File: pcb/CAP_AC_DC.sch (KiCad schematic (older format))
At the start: 6 parts

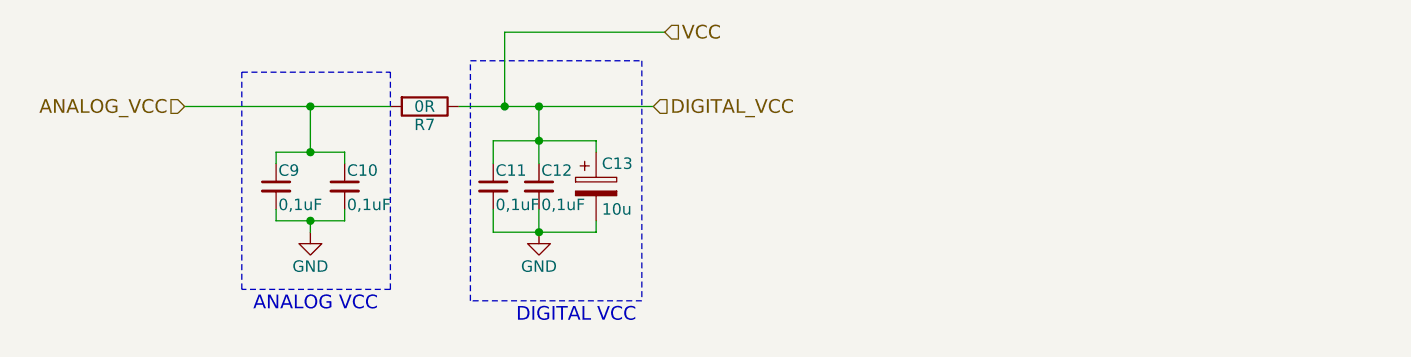
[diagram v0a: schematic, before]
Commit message: Clean up Kicad and TCC
Some changes in the
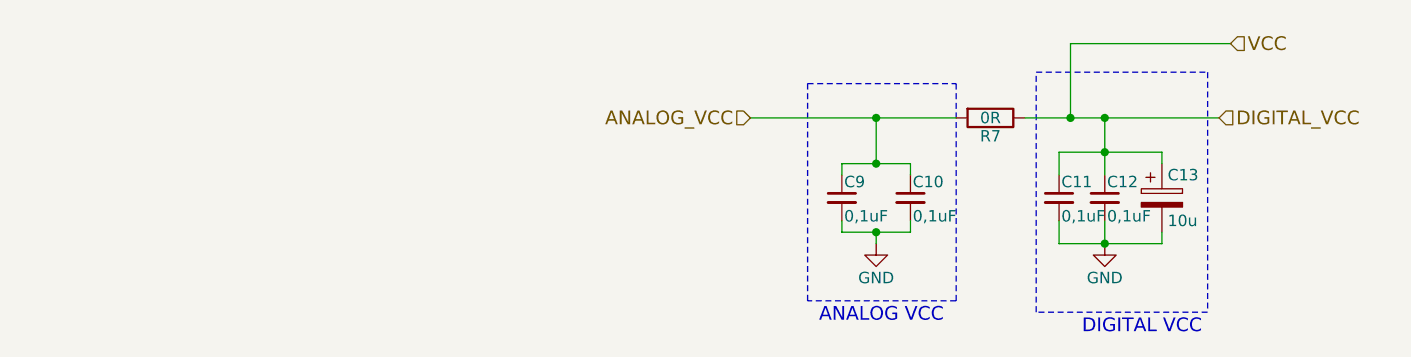
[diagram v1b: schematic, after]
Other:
- moved on the sheet: C10, C11, C12, C13, C9, R7
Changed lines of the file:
@@
 encoding utf-8
 Sheet 3 10
-Title ""
+Title "Capacitor Bank Schematic"
 Date ""
-Rev ""
-Comp ""
+Rev "1"
+Comp "Universidade de Brasília - Campus Gama"
 Comment1 ""
 Comment2 ""
@@
 L Device:C_Small C9
 U 1 1 5B1CC325
-P 3000 3650
-F 0 "C9" H 3010 3720 50  0000 L CNN
-F 1 "0,1uF" H 3010 3570 50  0000 L CNN
-F 2 "Capacitors_SMD:C_1206" H 3000 3650 50  0001 C CNN
-F 3 "https://www.digikey.com/product-detail/en/yageo/CC1206KRX7R9BB104/311-1179-1-ND/303089" H 3000 3650 50  0001 C CNN
-	1    3000 3650
+P 5475 3700
+F 0 "C9" H 5485 3770 50  0000 L CNN
+F 1 "0,1uF" H 5485 3620 50  0000 L CNN
+F 2 "Capacitors_SMD:C_1206" H 5475 3700 50  0001 C CNN
+F 3 "https://www.digikey.com/product-detail/en/yageo/CC1206KRX7R9BB104/311-1179-1-ND/303089" H 5475 3700 50  0001 C CNN
+	1    5475 3700
 	1    0    0    -1
 $EndComp
@@
 L Device:CP C13
 U 1 1 5B1CC377
-P 4400 3650
-F 0 "C13" H 4425 3750 50  0000 L CNN
-F 1 "10u" H 4425 3550 50  0000 L CNN
-F 2 "Capacitors_SMD:C_1206" H 4438 3500 50  0001 C CNN
-F 3 "https://www.digikey.com/product-detail/en/avx-corporation/TAJA106K006RNJ/478-1653-1-ND/564685" H 4400 3650 50  0001 C CNN
-	1    4400 3650
+P 6875 3700
+F 0 "C13" H 6900 3800 50  0000 L CNN
+F 1 "10u" H 6900 3600 50  0000 L CNN
+F 2 "Capacitors_SMD:C_1206" H 6913 3550 50  0001 C CNN
+F 3 "https://www.digikey.com/product-detail/en/avx-corporation/TAJA106K006RNJ/478-1653-1-ND/564685" H 6875 3700 50  0001 C CNN
+	1    6875 3700
 	1    0    0    -1
 $EndComp
@@
 L Device:C_Small C10
 U 1 1 5B1CC4B7
-P 3300 3650
-F 0 "C10" H 3310 3720 50  0000 L CNN
-F 1 "0,1uF" H 3310 3570 50  0000 L CNN
-F 2 "Capacitors_SMD:C_1206" H 3300 3650 50  0001 C CNN
-F 3 "https://www.digikey.com/product-detail/en/yageo/CC1206KRX7R9BB104/311-1179-1-ND/303089" H 3300 3650 50  0001 C CNN
-	1    3300 3650
+P 5775 3700
+F 0 "C10" H 5785 3770 50  0000 L CNN
+F 1 "0,1uF" H 5785 3620 50  0000 L CNN
+F 2 "Capacitors_SMD:C_1206" H 5775 3700 50  0001 C CNN
+F 3 "https://www.digikey.com/product-detail/en/yageo/CC1206KRX7R9BB104/311-1179-1-ND/303089" H 5775 3700 50  0001 C CNN
+	1    5775 3700
 	1    0    0    -1
 $EndComp
 Wire Wire Line
-	3000 3550 3000 3500
+	5475 3600 5475 3550
 Wire Wire Line
-	3000 3500 3150 3500
+	5475 3550 5625 3550
 Wire Wire Line
-	3300 3500 3300 3550
+	5775 3550 5775 3600
 Wire Wire Line
-	3300 3750 3300 3800
+	5775 3800 5775 3850
 Wire Wire Line
-	3300 3800 3150 3800
+	5775 3850 5625 3850
 Wire Wire Line
-	3000 3800 3000 3750
+	5475 3850 5475 3800
 $Comp
 L power:GND #PWR05
 U 1 1 5B1CC4EE
-P 3150 3850
-F 0 "#PWR05" H 3150 3600 50  0001 C CNN
-F 1 "GND" H 3150 3700 50  0000 C CNN
-F 2 "" H 3150 3850 50  0001 C CNN
-F 3 "" H 3150 3850 50  0001 C CNN
-	1    3150 3850
+P 5625 3900
+F 0 "#PWR05" H 5625 3650 50  0001 C CNN
+F 1 "GND" H 5625 3750 50  0000 C CNN
+F 2 "" H 5625 3900 50  0001 C CNN
+F 3 "" H 5625 3900 50  0001 C CNN
+	1    5625 3900
 	1    0    0    -1
 $EndComp
@@
 L Device:C_Small C11
 U 1 1 5B1CC509
-P 3950 3650
-F 0 "C11" H 3960 3720 50  0000 L CNN
-F 1 "0,1uF" H 3960 3570 50  0000 L CNN
-F 2 "Capacitors_SMD:C_1206" H 3950 3650 50  0001 C CNN
-F 3 "https://www.digikey.com/product-detail/en/yageo/CC1206KRX7R9BB104/311-1179-1-ND/303089" H 3950 3650 50  0001 C CNN
-	1    3950 3650
+P 6425 3700
+F 0 "C11" H 6435 3770 50  0000 L CNN
+F 1 "0,1uF" H 6435 3620 50  0000 L CNN
+F 2 "Capacitors_SMD:C_1206" H 6425 3700 50  0001 C CNN
+F 3 "https://www.digikey.com/product-detail/en/yageo/CC1206KRX7R9BB104/311-1179-1-ND/303089" H 6425 3700 50  0001 C CNN
+	1    6425 3700
 	1    0    0    -1
 $EndComp
@@
 L Device:C_Small C12
 U 1 1 5B1CC58F
-P 4150 3650
-F 0 "C12" H 4160 3720 50  0000 L CNN
-F 1 "0,1uF" H 4160 3570 50  0000 L CNN
-F 2 "Capacitors_SMD:C_1206" H 4150 3650 50  0001 C CNN
-F 3 "https://www.digikey.com/product-detail/en/yageo/CC1206KRX7R9BB104/311-1179-1-ND/303089" H 4150 3650 50  0001 C CNN
-	1    4150 3650
+P 6625 3700
+F 0 "C12" H 6635 3770 50  0000 L CNN
+F 1 "0,1uF" H 6635 3620 50  0000 L CNN
+F 2 "Capacitors_SMD:C_1206" H 6625 3700 50  0001 C CNN
+F 3 "https://www.digikey.com/product-detail/en/yageo/CC1206KRX7R9BB104/311-1179-1-ND/303089" H 6625 3700 50  0001 C CNN
+	1    6625 3700
 	1    0    0    -1
 $EndComp
 Wire Wire Line
-	4400 3450 4400 3500
+	6875 3500 6875 3550
 Wire Wire Line
-	3950 3450 4150 3450
+	6425 3500 6625 3500
 Wire Wire Line
-	3950 3450 3950 3550
+	6425 3500 6425 3600
 Wire Wire Line
-	4150 3300 4150 3450
-Connection ~ 4150 3450
+	6625 3350 6625 3500
+Connection ~ 6625 3500
 Wire Wire Line
-	3950 3750 3950 3850
+	6425 3800 6425 3900
 Wire Wire Line
-	3950 3850 4150 3850
+	6425 3900 6625 3900
 Wire Wire Line
-	4400 3850 4400 3800
+	6875 3900 6875 3850
 Wire Wire Line
-	4150 3750 4150 3850
-Connection ~ 4150 3850
+	6625 3800 6625 3900
+Connection ~ 6625 3900
 $Comp
 L power:GND #PWR06
 U 1 1 5B1CC5FE
-P 4150 3850
-F 0 "#PWR06" H 4150 3600 50  0001 C CNN
-F 1 "GND" H 4150 3700 50  0000 C CNN
-F 2 "" H 4150 3850 50  0001 C CNN
-F 3 "" H 4150 3850 50  0001 C CNN
-	1    4150 3850
+P 6625 3900
+F 0 "#PWR06" H 6625 3650 50  0001 C CNN
+F 1 "GND" H 6625 3750 50  0000 C CNN
+F 2 "" H 6625 3900 50  0001 C CNN
+F 3 "" H 6625 3900 50  0001 C CNN
+	1    6625 3900
 	1    0    0    -1
 $EndComp
@@
 L Device:R R7
 U 1 1 5B1CC61A
-P 3650 3300
-F 0 "R7" V 3730 3300 50  0000 C CNN
-F 1 "0R" V 3650 3300 50  0000 C CNN
-F 2 "Resistors_SMD:R_1206" V 3580 3300 50  0001 C CNN
-F 3 "https://www.digikey.com/product-detail/en/stackpole-electronics-inc/RMCF1206ZT0R00/RMCF1206ZT0R00TR-ND/1756906" H 3650 3300 50  0001 C CNN
-	1    3650 3300
+P 6125 3350
+F 0 "R7" V 6205 3350 50  0000 C CNN
+F 1 "0R" V 6125 3350 50  0000 C CNN
+F 2 "Resistors_SMD:R_1206" V 6055 3350 50  0001 C CNN
+F 3 "https://www.digikey.com/product-detail/en/stackpole-electronics-inc/RMCF1206ZT0R00/RMCF1206ZT0R00TR-ND/1756906" H 6125 3350 50  0001 C CNN
+	1    6125 3350
 	0    1    1    0
 $EndComp
 Wire Wire Line
-	2600 3300 3150 3300
+	5075 3350 5625 3350
 Wire Wire Line
-	3150 3300 3150 3500
-Connection ~ 3150 3500
+	5625 3350 5625 3550
+Connection ~ 5625 3550
 Wire Wire Line
-	3800 3300 4000 3300
+	6275 3350 6475 3350
 Wire Notes Line
-	2850 3150 3500 3150
+	5325 3200 5975 3200
 Wire Notes Line
-	3500 3150 3500 4100
+	5975 3200 5975 4150
 Wire Notes Line
-	3500 4100 2850 4100
+	5975 4150 5325 4150
 Wire Notes Line
-	2850 4100 2850 3150
+	5325 4150 5325 3200
 Wire Notes Line
-	3850 3100 4600 3100
+	6325 3150 7075 3150
 Wire Notes Line
-	4600 3100 4600 4150
+	7075 3150 7075 4200
 Wire Notes Line
-	4600 4150 3850 4150
+	7075 4200 6325 4200
 Wire Notes Line
-	3850 4150 3850 3100
-Text Notes 4050 4250 0    60   ~ 0
+	6325 4200 6325 3150
+Text Notes 6525 4300 0    60   ~ 0
 DIGITAL VCC\n
-Text Notes 2900 4200 0    60   ~ 0
+Text Notes 5375 4250 0    60   ~ 0
 ANALOG VCC\n
-Text HLabel 2600 3300 0    60   Input ~ 0
+Text HLabel 5075 3350 0    60   Input ~ 0
 ANALOG_VCC
-Connection ~ 3150 3300
-Text HLabel 4650 3300 2    60   Input ~ 0
+Connection ~ 5625 3350
+Text HLabel 7125 3350 2    60   Input ~ 0
 DIGITAL_VCC
-Connection ~ 4150 3300
-Text HLabel 4700 2975 2    60   Input ~ 0
+Connection ~ 6625 3350
+Text HLabel 7175 3025 2    60   Input ~ 0
 VCC
 Wire Wire Line
-	4000 2975 4000 3300
-Connection ~ 4000 3300
+	6475 3025 6475 3350
+Connection ~ 6475 3350
 Wire Wire Line
-	4700 2975 4000 2975
+	7175 3025 6475 3025
 Wire Wire Line
-	3150 3850 3150 3800
-Connection ~ 3150 3800
+	5625 3900 5625 3850
+Connection ~ 5625 3850
 Wire Wire Line
-	4150 3450 4400 3450
+	6625 3500 6875 3500
 Wire Wire Line
-	4150 3450 4150 3550
+	6625 3500 6625 3600
 Wire Wire Line
-	4150 3850 4400 3850
+	6625 3900 6875 3900
 Wire Wire Line
-	3150 3500 3300 3500
+	5625 3550 5775 3550
 Wire Wire Line
-	3150 3300 3500 3300
+	5625 3350 5975 3350
 Wire Wire Line
-	4150 3300 4650 3300
+	6625 3350 7125 3350
 Wire Wire Line
-	4000 3300 4150 3300
+	6475 3350 6625 3350
 Wire Wire Line
-	3150 3800 3000 3800
+	5625 3850 5475 3850
 $EndSCHEMATC
